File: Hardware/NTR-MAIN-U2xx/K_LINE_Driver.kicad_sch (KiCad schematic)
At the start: 11 parts, among them U5 74AHC1G08SE-7, U6 TJA1027T

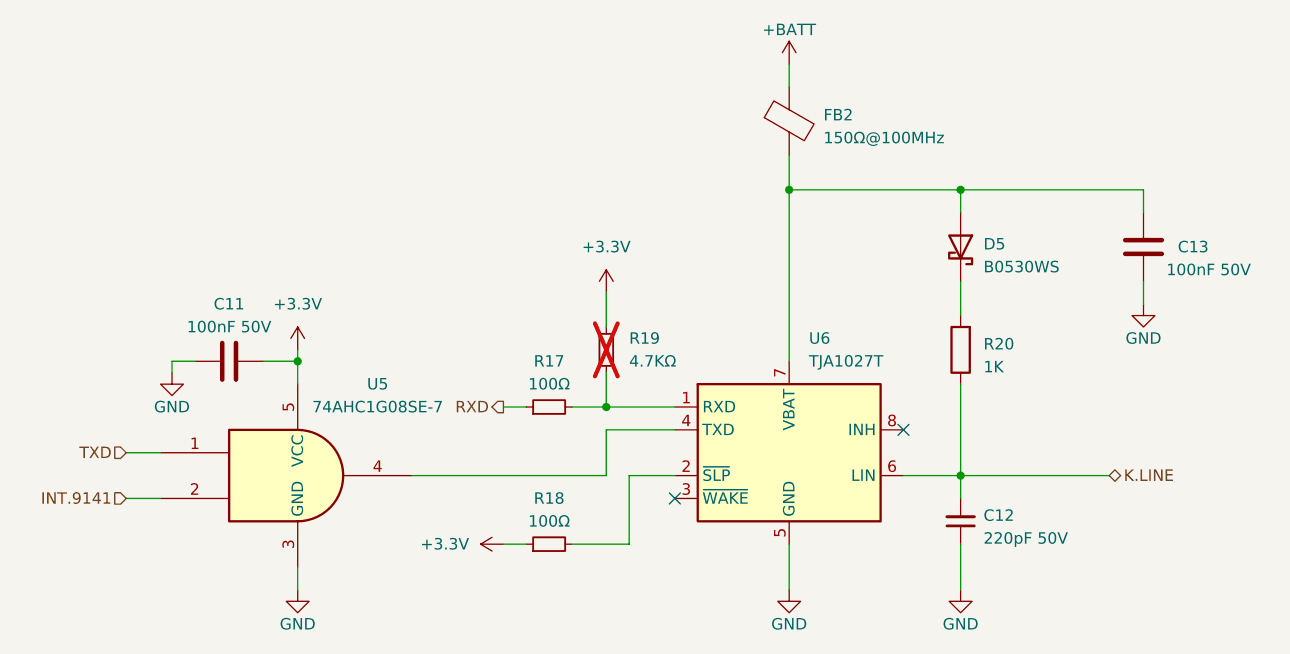
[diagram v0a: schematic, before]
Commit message: update boot and app
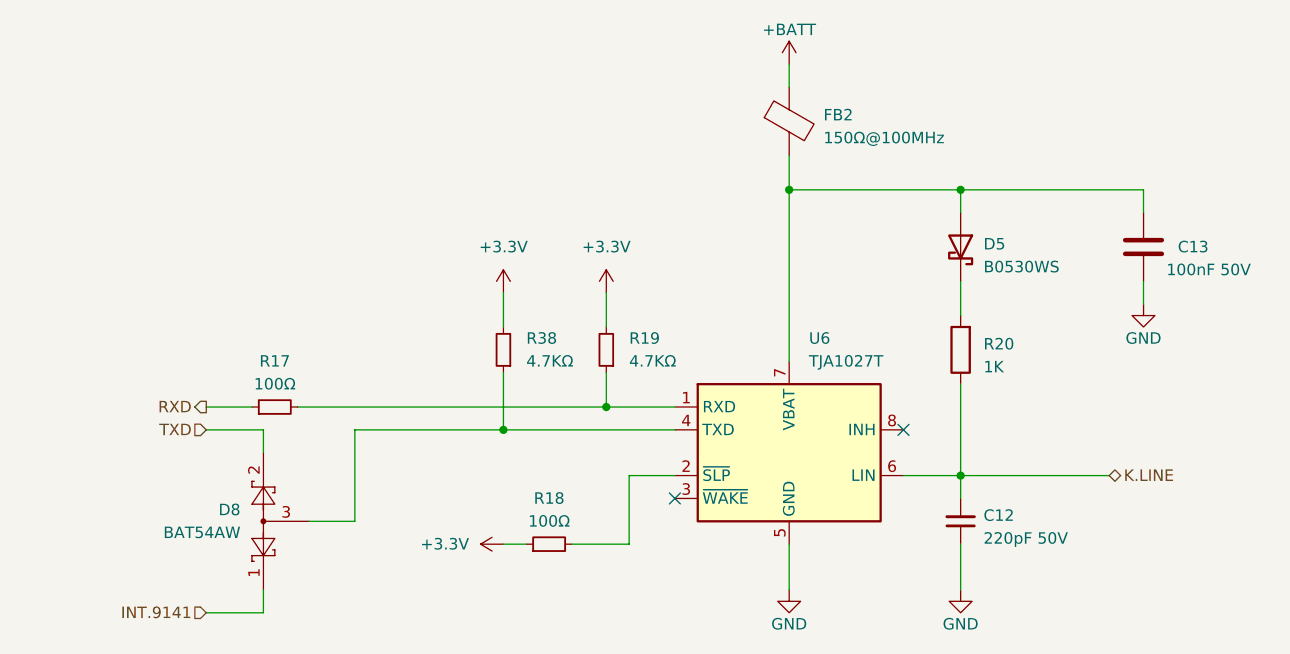
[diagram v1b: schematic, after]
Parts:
- removed C11: 100nF 50V, Capacitor_SMD:C_0402_1005Metric, symbol Device:C
- removed U5: 74AHC1G08SE-7, Package_TO_SOT_SMD:SOT-353_SC-70-5, symbol 74xGxx:74AHC1G08
- added D8: BAT54AW, Package_TO_SOT_SMD:SOT-323_SC-70, symbol Diode:BAT54AW
- added R38: 4.7KΩ, Resistor_SMD:R_0402_1005Metric, symbol Device:R_Small
- R19: now fitted; now in the parts list
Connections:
- net +3.3V: now also R38.2
- net INT.9141: now also D8.1
- net TXD: now also D8.2
- net at U6.4 (TXD): now also D8.3, R38.1
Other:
- moved on the sheet: R17
